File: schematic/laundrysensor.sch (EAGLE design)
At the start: 15 parts, among them Q1 2N3904, Q2 2N3904

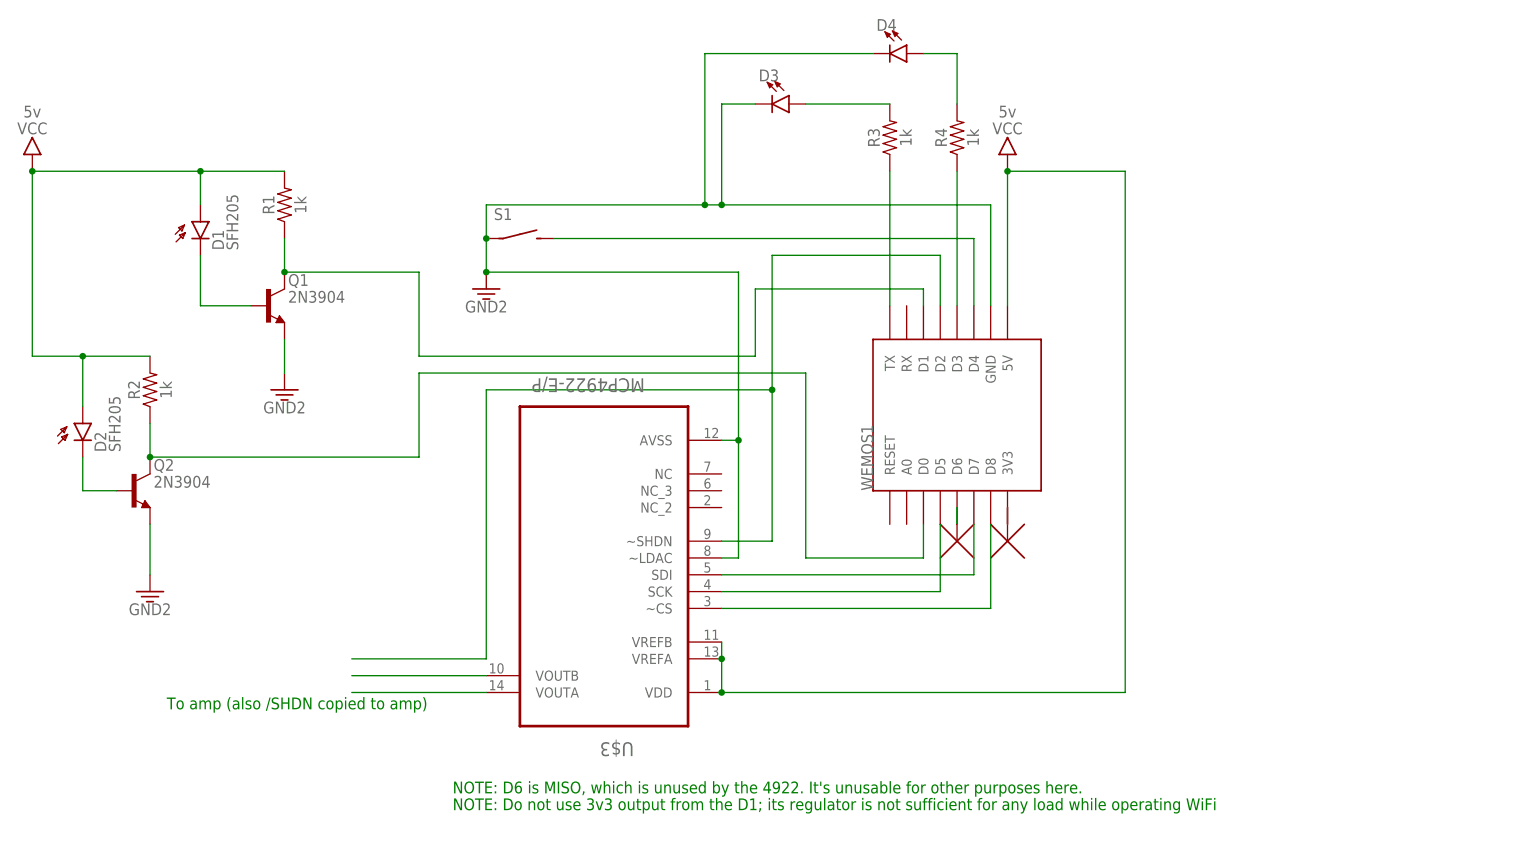
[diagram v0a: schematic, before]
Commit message: working on i2s audio methods...
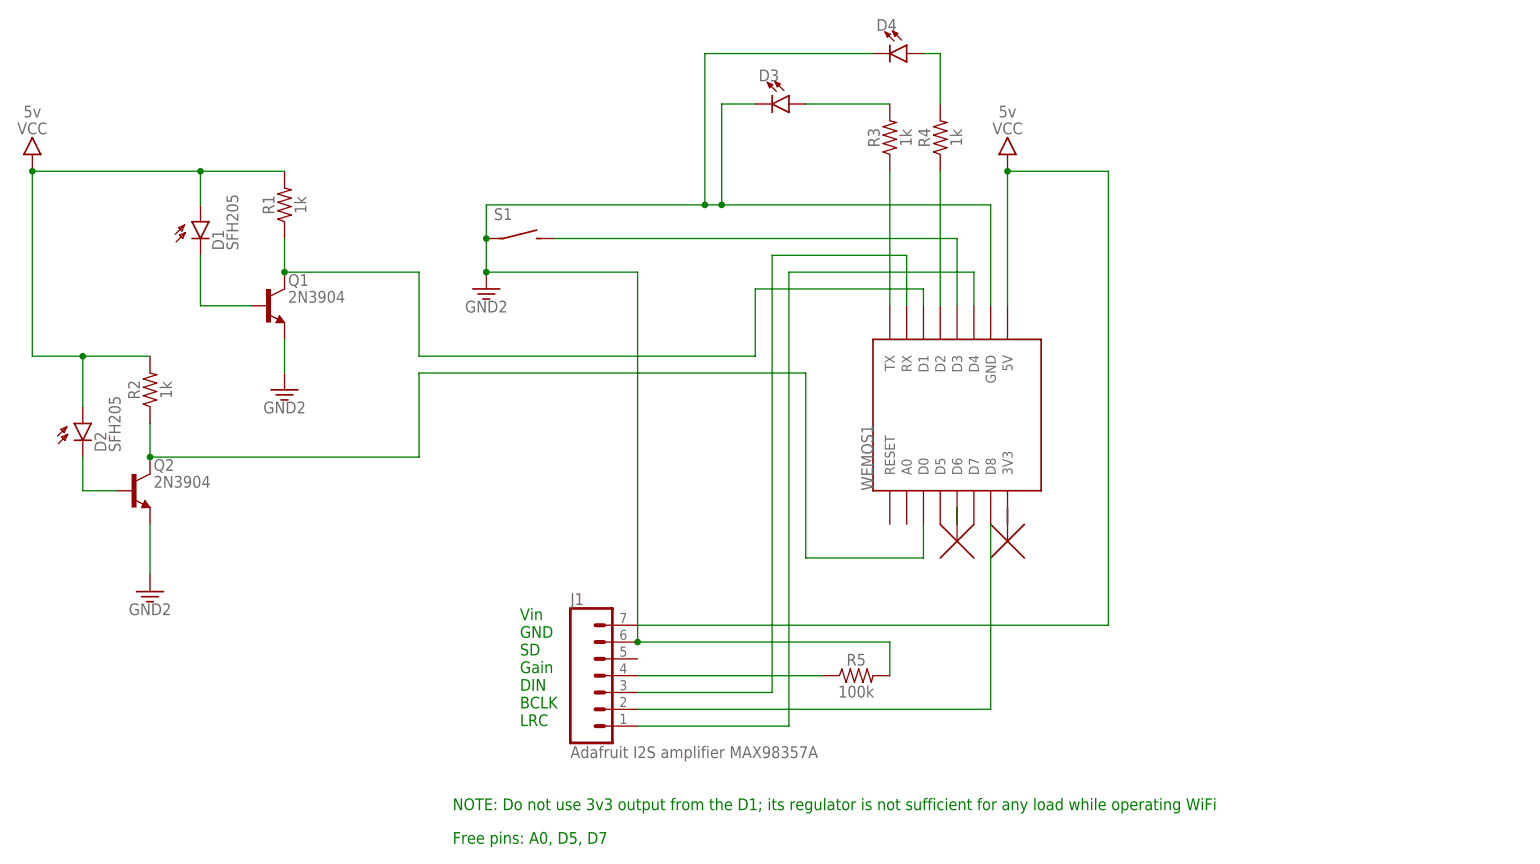
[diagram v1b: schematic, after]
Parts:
- removed U$3: MCP4922-E/P, MCP4922-E_P:MCP4922-E/P
- added J1: Adafruit I2S amplifier MAX98357A, SparkFun-Connectors:CONN_07
- added R5: 100k, SparkFun-Resistors:100KOHM-HORIZ-1/4W-1%
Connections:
- removed net N$16: U$3.VOUTA
- removed net N$17: U$3.VOUTB
- net 3.3V: now also J1.6, R5.2; no longer U$3.AVSS, U$3.~LDAC
- net N$10: now also J1.1, WEMOS1.D4; no longer R4.1, WEMOS1.D3
- net N$2: now also R4.1, WEMOS1.D2; no longer U$3.SCK, WEMOS1.D5
- net N$4: now also WEMOS1.D3; no longer WEMOS1.D4
- net N$7: now also J1.4, R5.1; no longer U$3.SDI, WEMOS1.D7
- net N$8: now also J1.3, WEMOS1.RX; no longer U$3.~CS, WEMOS1.D8
- net N$9: now also J1.2, WEMOS1.D8; no longer U$3.~SHDN, WEMOS1.D2
- net VCC: now also J1.7; no longer U$3.VDD, U$3.VREFA, U$3.VREFB
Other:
- note added: "Free pins: A0, D5, D7"
- note added: "Vin GND SD Gain DIN BCLK LRC"
- note removed: "NOTE: D6 is MISO, which is unused by the 4922. It's unusable for other purposes here."
- note removed: "To amp (also /SHDN copied to amp)"
- moved on the sheet: R4
